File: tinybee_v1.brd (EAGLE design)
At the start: 47.6 x 27.8 mm, 22 parts, among them U1 ATTINY85-20S

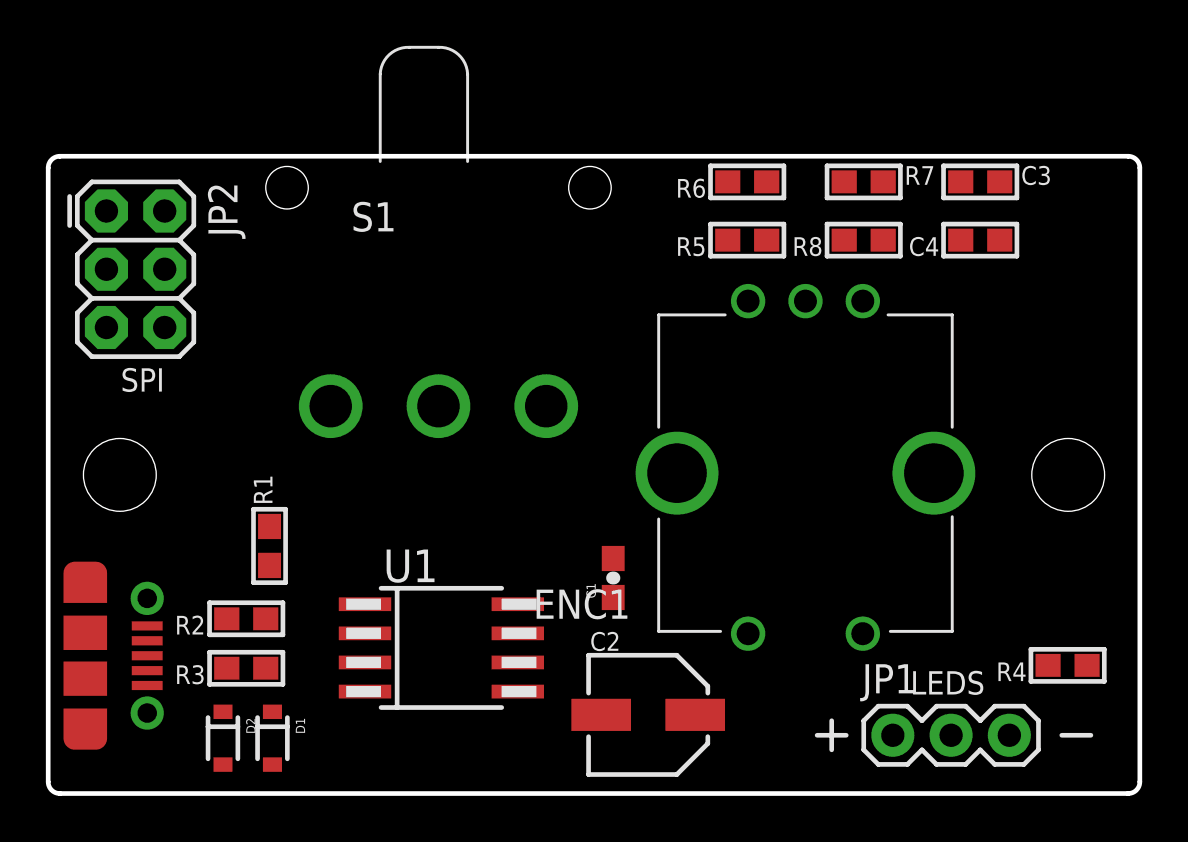
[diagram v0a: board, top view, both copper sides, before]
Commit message: moved a few pieces
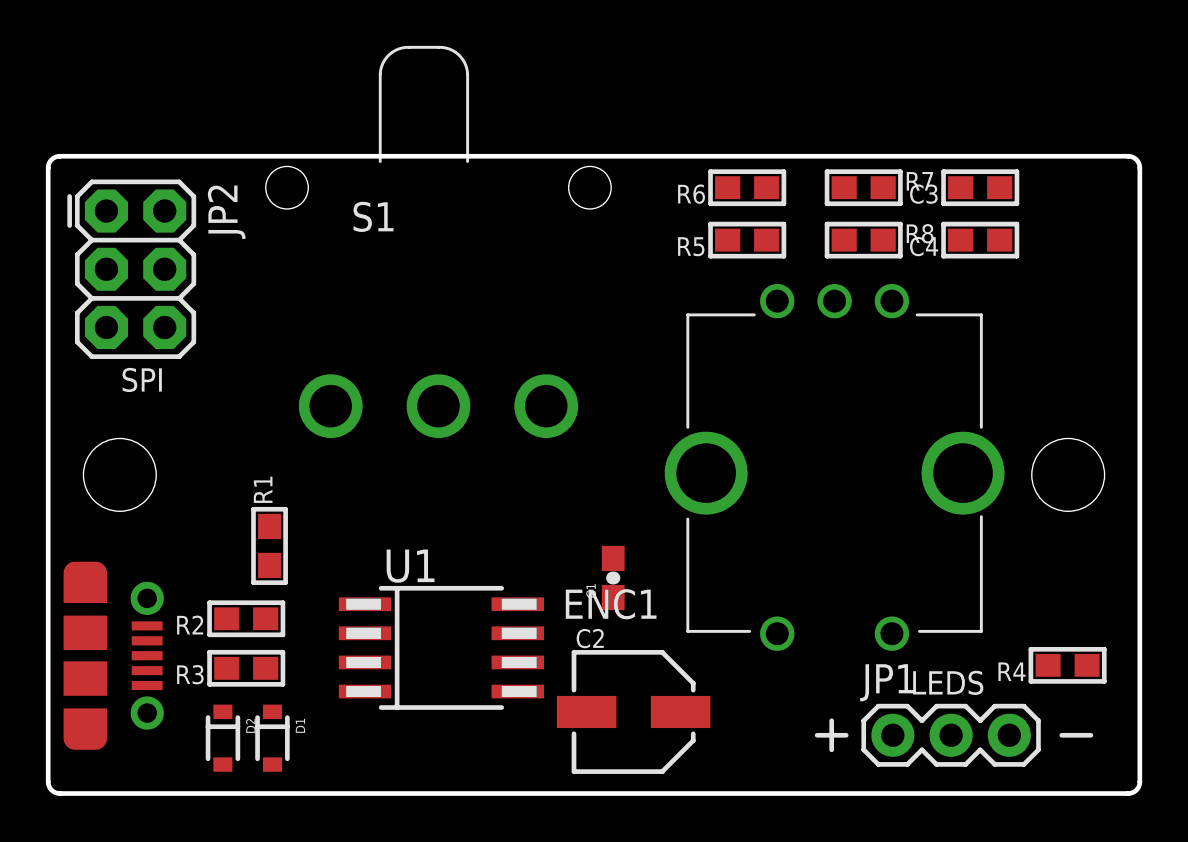
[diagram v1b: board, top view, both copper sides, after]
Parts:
- moved ENC1 1.27 mm to (34.3, 14.0)
- moved C2 0.65 mm to (25.5, 3.56)
- moved C3 0.25 mm to (40.6, 26.4), turned to 180 degrees
- moved R6 0.25 mm to (30.5, 26.4)
- moved R7 0.25 mm to (35.6, 26.4)
- turned R8 to 0 degrees
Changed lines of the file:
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@@
 <attribute name="PROD_ID" value="CAP-00810" x="24.638" y="9.398" size="1.778" layer="27" rot="R90" display="off"/>
 </element>
-<element name="C2" library="microbuilder" package="PANASONIC_C" value="47uF" x="26.162" y="3.429"/>
-<element name="C3" library="microbuilder" package="0603" value="0.1uF" x="40.64" y="26.67"/>
+<element name="C2" library="microbuilder" package="PANASONIC_C" value="47uF" x="25.527" y="3.556"/>
+<element name="C3" library="microbuilder" package="0603" value="0.1uF" x="40.64" y="26.416" rot="R180"/>
 <element name="C4" library="microbuilder" package="0603" value="0.1uF" x="40.64" y="24.13" rot="R180"/>
 <element name="D1" library="SparkFun-DiscreteSemi" package="SOD-323" value="3.6V" x="9.779" y="2.413" rot="R270">
@@
 <element name="JP1" library="SparkFun-Connectors" package="1X03" value="LEDS" x="36.83" y="2.54"/>
 <element name="R5" library="microbuilder" package="0603" value="10k" x="30.48" y="24.13" rot="R180"/>
-<element name="R6" library="microbuilder" package="0603" value="10k" x="30.48" y="26.67" rot="R180"/>
-<element name="R7" library="microbuilder" package="0603" value="10k" x="35.56" y="26.67"/>
-<element name="R8" library="microbuilder" package="0603" value="10k" x="35.56" y="24.13" rot="R180"/>
+<element name="R6" library="microbuilder" package="0603" value="10k" x="30.48" y="26.416" rot="R180"/>
+<element name="R7" library="microbuilder" package="0603" value="10k" x="35.56" y="26.416"/>
+<element name="R8" library="microbuilder" package="0603" value="10k" x="35.56" y="24.13"/>
 <element name="U1" library="_hhn_attiny25_45_85" package="SOIC8_EIAJ_208MIL" value="ATTINY85-20S" x="17.145" y="6.35" rot="R270"/>
 <element name="USB" library="GeekAmmo" package="USB-MICRO-MOLEX-105017-0001" value="USB-CON-5PIN-105017-0001" x="4.318" y="8.509" rot="R270"/>
@@
 <element name="R2" library="microbuilder" package="0603" value="68R" x="8.636" y="7.62" rot="R180"/>
 <element name="R4" library="microbuilder" package="0603" value="220R" x="44.45" y="5.588" rot="R180"/>
-<element name="ENC1" library="Custom" package="ROTARY-ENCODER-PEC12R" value="" x="33.02" y="13.97" rot="R180"/>
+<element name="ENC1" library="Custom" package="ROTARY-ENCODER-PEC12R" value="" x="34.29" y="13.97" rot="R180"/>
 <element name="U$1" library="Custom" package="FB-30" value="" x="0" y="0"/>
 <element name="S1" library="Custom" package="SWITCH-SPDT-RIGHTANGLE-500" value="" x="17.018" y="16.891"/>
@@
 <contactref element="U1" pad="8"/>
 <contactref element="C1" pad="1"/>
-<wire x1="34.71" y1="24.13" x2="36.41" y2="26.67" width="0" layer="19" extent="1-1"/>
-<wire x1="24.638" y1="8.548" x2="34.71" y2="24.13" width="0" layer="19" extent="1-1"/>
+<wire x1="36.41" y1="24.13" x2="36.41" y2="26.416" width="0" layer="19" extent="1-1"/>
+<wire x1="24.638" y1="8.548" x2="36.41" y2="24.13" width="0" layer="19" extent="1-1"/>
 <wire x1="20.475" y1="8.255" x2="24.638" y2="8.548" width="0" layer="19" extent="1-1"/>
-<wire x1="28.212" y1="3.429" x2="24.638" y2="8.548" width="0" layer="19" extent="1-1"/>
-<wire x1="36.83" y1="2.54" x2="28.212" y2="3.429" width="0" layer="19" extent="1-1"/>
+<wire x1="27.577" y1="3.556" x2="24.638" y2="8.548" width="0" layer="19" extent="1-1"/>
+<wire x1="36.83" y1="2.54" x2="27.577" y2="3.556" width="0" layer="19" extent="1-1"/>
 <wire x1="17.018" y1="16.891" x2="20.475" y2="8.255" width="0" layer="19" extent="1-1"/>
 <wire x1="9.652" y1="11.645" x2="17.018" y2="16.891" width="0" layer="19" extent="1-1"/>
@@
 <contactref element="ENC1" pad="C"/>
 <contactref element="C1" pad="2"/>
-<wire x1="41.49" y1="24.13" x2="39.79" y2="26.67" width="0" layer="19" extent="1-1"/>
-<wire x1="33.02" y1="21.47" x2="39.79" y2="26.67" width="0" layer="19" extent="1-1"/>
-<wire x1="24.638" y1="10.248" x2="33.02" y2="21.47" width="0" layer="19" extent="1-1"/>
-<wire x1="24.112" y1="3.429" x2="24.638" y2="10.248" width="0" layer="19" extent="1-1"/>
-<wire x1="13.815" y1="4.445" x2="24.112" y2="3.429" width="0" layer="19" extent="1-1"/>
+<wire x1="41.49" y1="24.13" x2="41.49" y2="26.416" width="0" layer="19" extent="1-1"/>
+<wire x1="34.29" y1="21.47" x2="41.49" y2="24.13" width="0" layer="19" extent="1-1"/>
+<wire x1="36.79" y1="6.97" x2="34.29" y2="21.47" width="0" layer="19" extent="1-1"/>
+<wire x1="41.91" y1="2.54" x2="36.79" y2="6.97" width="0" layer="19" extent="1-1"/>
+<wire x1="24.638" y1="10.248" x2="36.79" y2="6.97" width="0" layer="19" extent="1-1"/>
+<wire x1="23.477" y1="3.556" x2="24.638" y2="10.248" width="0" layer="19" extent="1-1"/>
+<wire x1="13.815" y1="4.445" x2="23.477" y2="3.556" width="0" layer="19" extent="1-1"/>
 <wire x1="9.779" y1="1.263" x2="13.815" y2="4.445" width="0" layer="19" extent="1-1"/>
 <wire x1="7.62" y1="1.263" x2="9.779" y2="1.263" width="0" layer="19" extent="1-1"/>
 <wire x1="4.318" y1="4.709" x2="7.62" y2="1.263" width="0" layer="19" extent="1-1"/>
-<wire x1="35.52" y1="6.97" x2="24.638" y2="10.248" width="0" layer="19" extent="1-1"/>
-<wire x1="41.91" y1="2.54" x2="35.52" y2="6.97" width="0" layer="19" extent="1-1"/>
 <wire x1="5.08" y1="20.32" x2="4.318" y2="4.709" width="0" layer="19" extent="1-1"/>
 </signal>
@@
 <contactref element="R2" pad="1"/>
 <contactref element="ENC1" pad="SW2"/>
-<wire x1="13.815" y1="6.985" x2="30.52" y2="6.97" width="0" layer="19" extent="1-1"/>
+<wire x1="13.815" y1="6.985" x2="31.79" y2="6.97" width="0" layer="19" extent="1-1"/>
 <wire x1="9.486" y1="7.62" x2="13.815" y2="6.985" width="0" layer="19" extent="1-1"/>
 </signal>
@@
 <contactref element="R7" pad="1"/>
 <contactref element="ENC1" pad="A"/>
-<wire x1="31.33" y1="26.67" x2="34.71" y2="26.67" width="0" layer="19" extent="1-1"/>
-<wire x1="35.52" y1="21.47" x2="34.71" y2="26.67" width="0" layer="19" extent="1-1"/>
+<wire x1="31.33" y1="26.416" x2="34.71" y2="26.416" width="0" layer="19" extent="1-1"/>
+<wire x1="36.79" y1="21.47" x2="34.71" y2="26.416" width="0" layer="19" extent="1-1"/>
 </signal>
 <signal name="N$8">
@@
 <contactref element="R8" pad="1"/>
 <contactref element="ENC1" pad="B"/>
-<wire x1="31.33" y1="24.13" x2="36.41" y2="24.13" width="0" layer="19" extent="1-1"/>
-<wire x1="30.52" y1="21.47" x2="31.33" y2="24.13" width="0" layer="19" extent="1-1"/>
+<wire x1="31.33" y1="24.13" x2="34.71" y2="24.13" width="0" layer="19" extent="1-1"/>
+<wire x1="31.79" y1="21.47" x2="31.33" y2="24.13" width="0" layer="19" extent="1-1"/>
 </signal>
 <signal name="N$11">
@@
 <contactref element="C3" pad="2"/>
 <contactref element="JP2" pad="4"/>
-<wire x1="29.63" y1="26.67" x2="41.49" y2="26.67" width="0" layer="19" extent="1-1"/>
-<wire x1="20.475" y1="4.445" x2="29.63" y2="26.67" width="0" layer="19" extent="1-1"/>
+<wire x1="29.63" y1="26.416" x2="39.79" y2="26.416" width="0" layer="19" extent="1-1"/>
+<wire x1="20.475" y1="4.445" x2="29.63" y2="26.416" width="0" layer="19" extent="1-1"/>
 <wire x1="5.08" y1="22.86" x2="20.475" y2="4.445" width="0" layer="19" extent="1-1"/>
 </signal>
